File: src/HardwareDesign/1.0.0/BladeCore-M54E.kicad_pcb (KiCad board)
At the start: 6 copper layers, 29 x 80.6 mm, 150 parts, among them IC1 RP2354B, IC10 SN74LVC1G97QDCKRQ1, IC2 AT24C256C-XHL-T, IC3 W25Q128JVPIQ, IC4 MCP6001RT, IC5 LM4040B30FTA, IC6 W5500, IC7 TPS74801DRCT, IC8 SN74LVC1G97QDCKRQ1, IC9 FSUSB42MUX, J1 MDT320M03001, J2 SM03B-SRSS-TB, J3 USB-TYPE-C-018, SW1 B3U-1000P, SW2 B3U-1000P, X1 12MHz 10pF, X2 25MHz 12pF

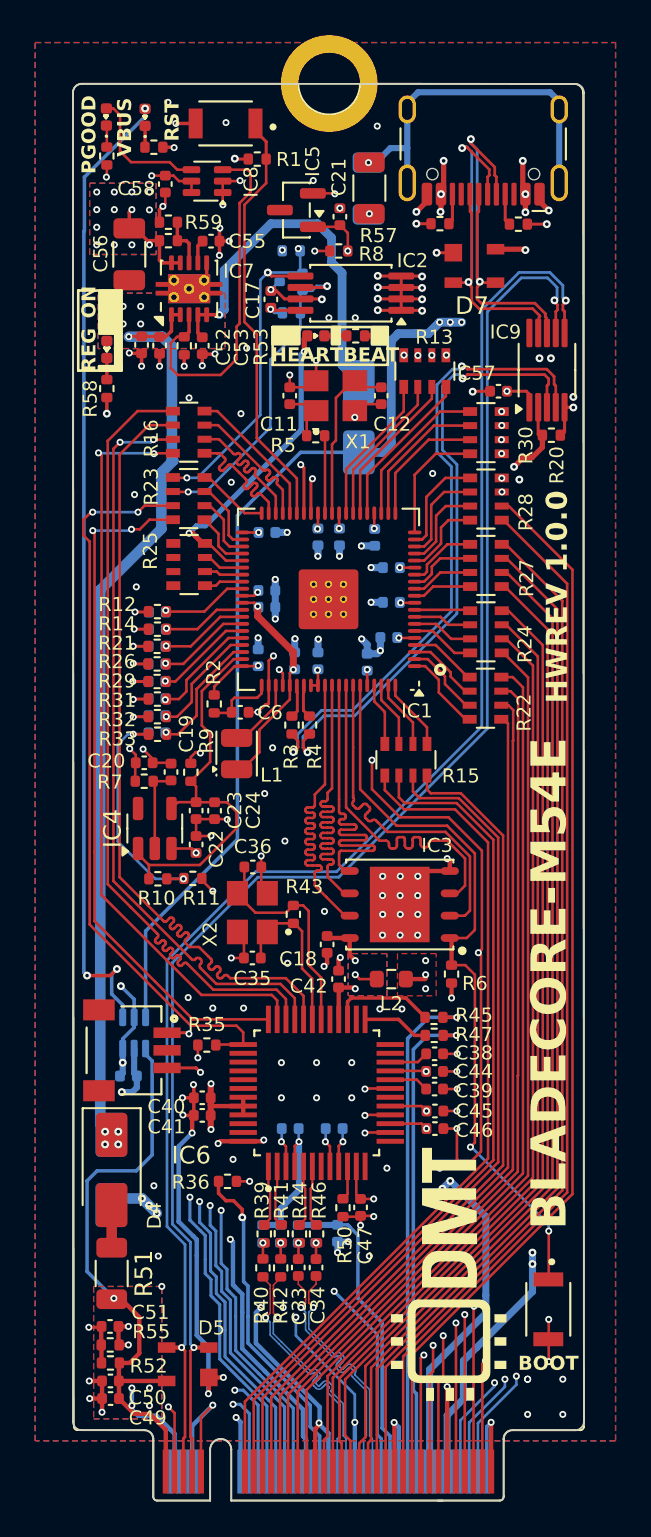
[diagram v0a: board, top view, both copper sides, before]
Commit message: update documentation
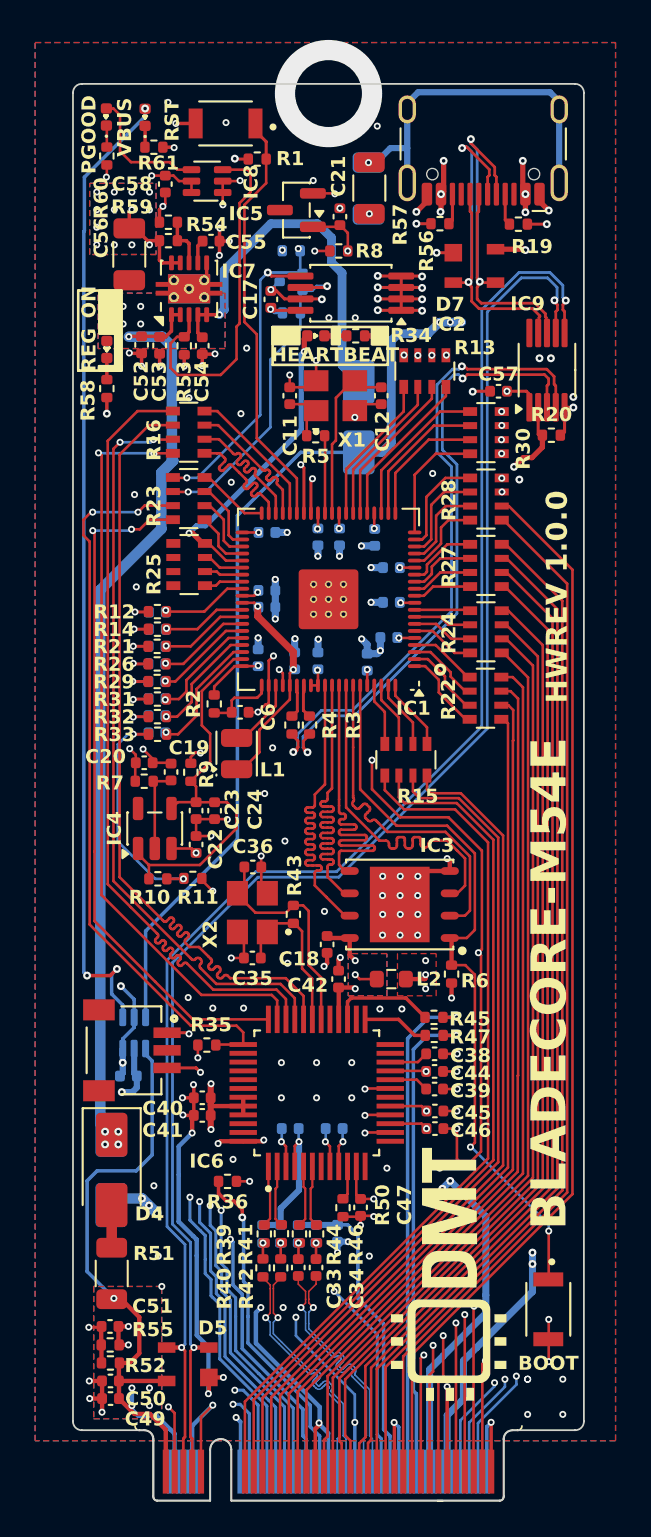
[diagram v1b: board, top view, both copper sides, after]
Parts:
- C1, C10, C11, C12, C13, C14, C15, C16, C17, C18, C19, C2, C20, C21, C22, C23, C24, C25, C26, C27, C28, C29, C3, C30, C31, C32, C33, C34, C35, C36, C37, C38, C39, C4, C40, C41, C42, C43, C44, C45, C46, C47, C48, C49, C5, C50, C51, C52, C53, C54, C55, C57, C58, C6, C60, C7, C8, C9: footprint Capacitor_SMD:C_0402_1005Metric -> DS_Capacitor:C_0402_1005Metric
- C56, C59: footprint Capacitor_SMD:C_1206_3216Metric -> DS_Capacitor:C_1206_3216Metric
- D10, D11, D3, D6: footprint LED_SMD:LED_0402_1005Metric -> DS_Opto:LED_0402_1005Metric
- J1: footprint DS_Connector:M.2-M-KEY_Card_2280 -> DS_Connector:M.2-M-KEY_Card_Plain
- R1, R10, R11, R12, R14, R17, R18, R19, R2, R20, R21, R26, R29, R3, R31, R32, R33, R34, R35, R36, R37, R38, R39, R4, R40, R41, R42, R43, R44, R45, R46, R47, R48, R49, R5, R50, R52, R53, R54, R55, R56, R58, R59, R6, R60, R61, R7, R8, R9: footprint Resistor_SMD:R_0402_1005Metric -> DS_Resistor:R_0402_1005Metric
- R13, R15, R16, R22, R23, R24, R25, R27, R28, R30: footprint Resistor_SMD:R_Array_Convex_4x0603 -> DS_Resistor:R_Array_Convex_4x0603
- R51, R57: footprint Resistor_SMD:R_1206_3216Metric -> DS_Resistor:R_1206_3216Metric
- moved J1 39.1 mm to (221.4, 164.6)
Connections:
- IC5 pad 3: (no net) -> unconnected-(IC5-NC-Pad3)
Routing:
- net GND: track 243.9 -> 244.0 mm, vias 164 -> 165
